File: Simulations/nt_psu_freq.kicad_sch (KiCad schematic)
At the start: 14 parts, among them Q1 DMP2008UFG

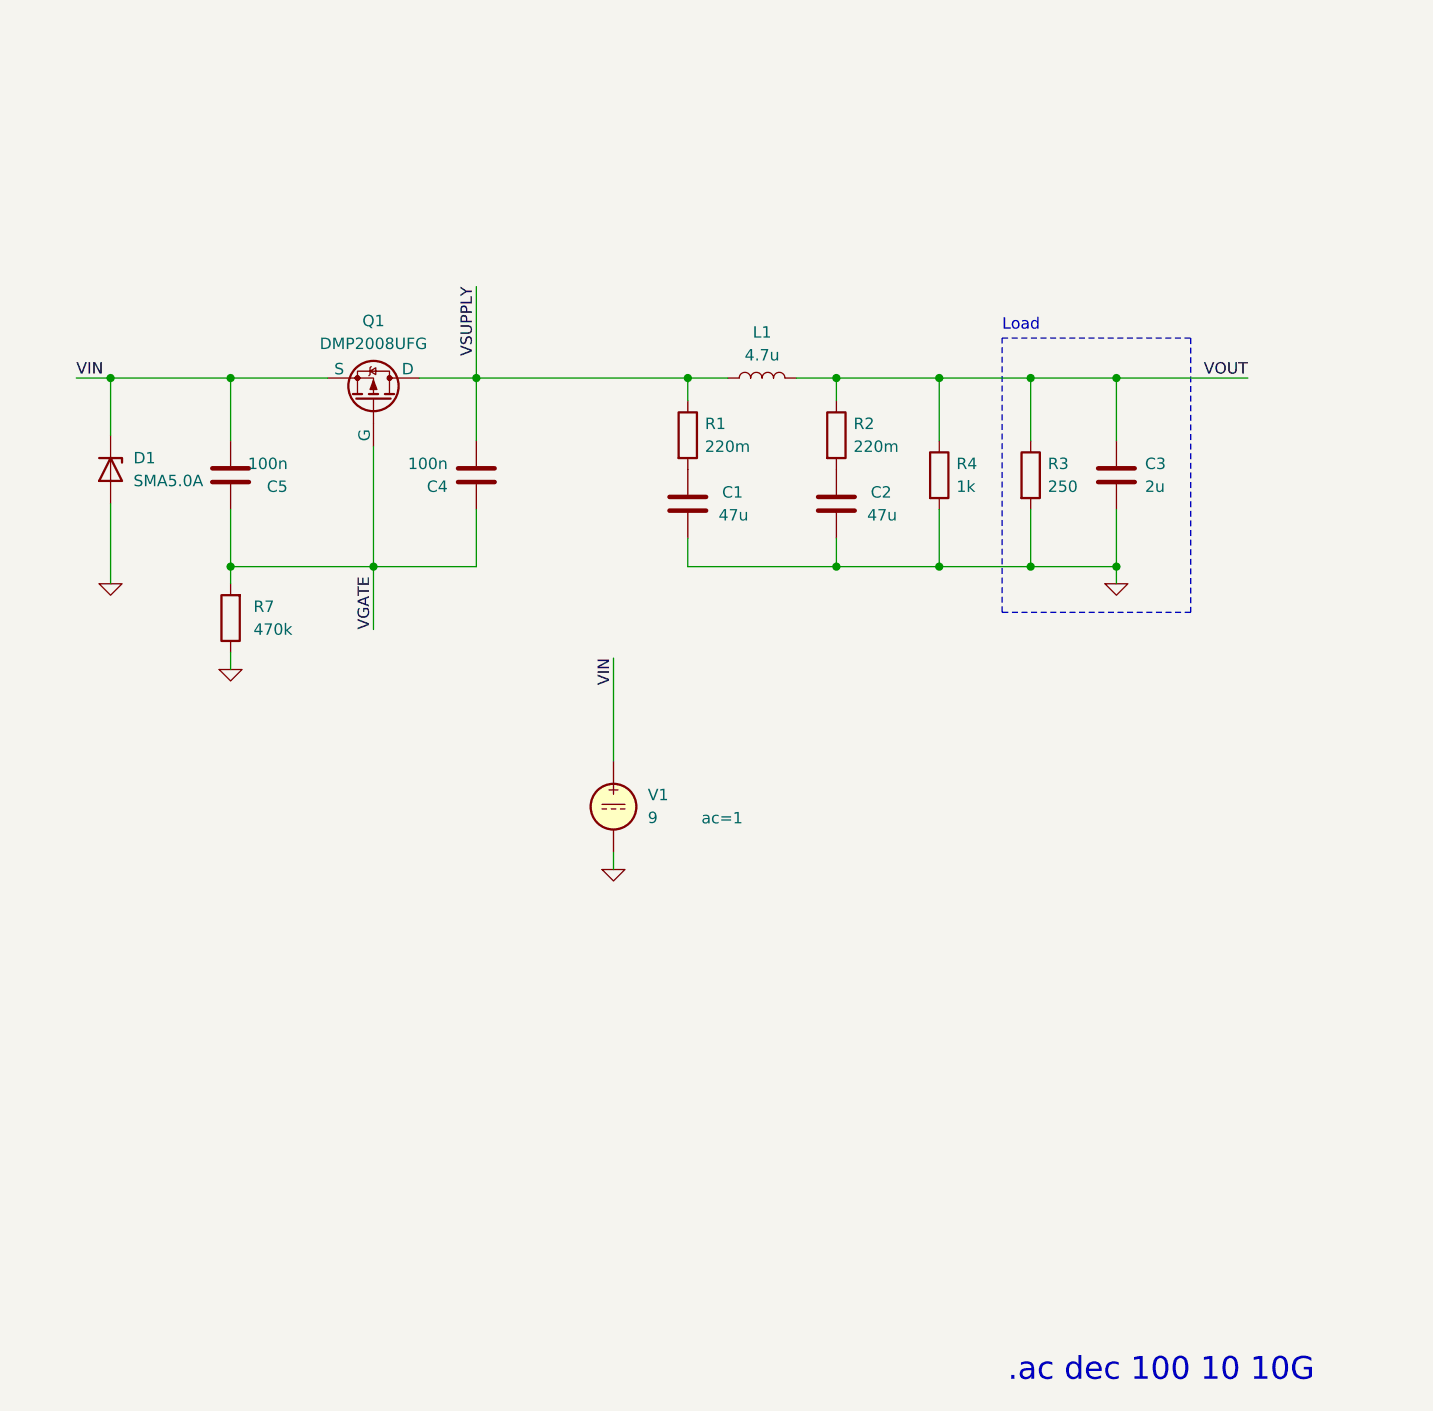
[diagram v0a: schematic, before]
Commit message: fine tuning before layout
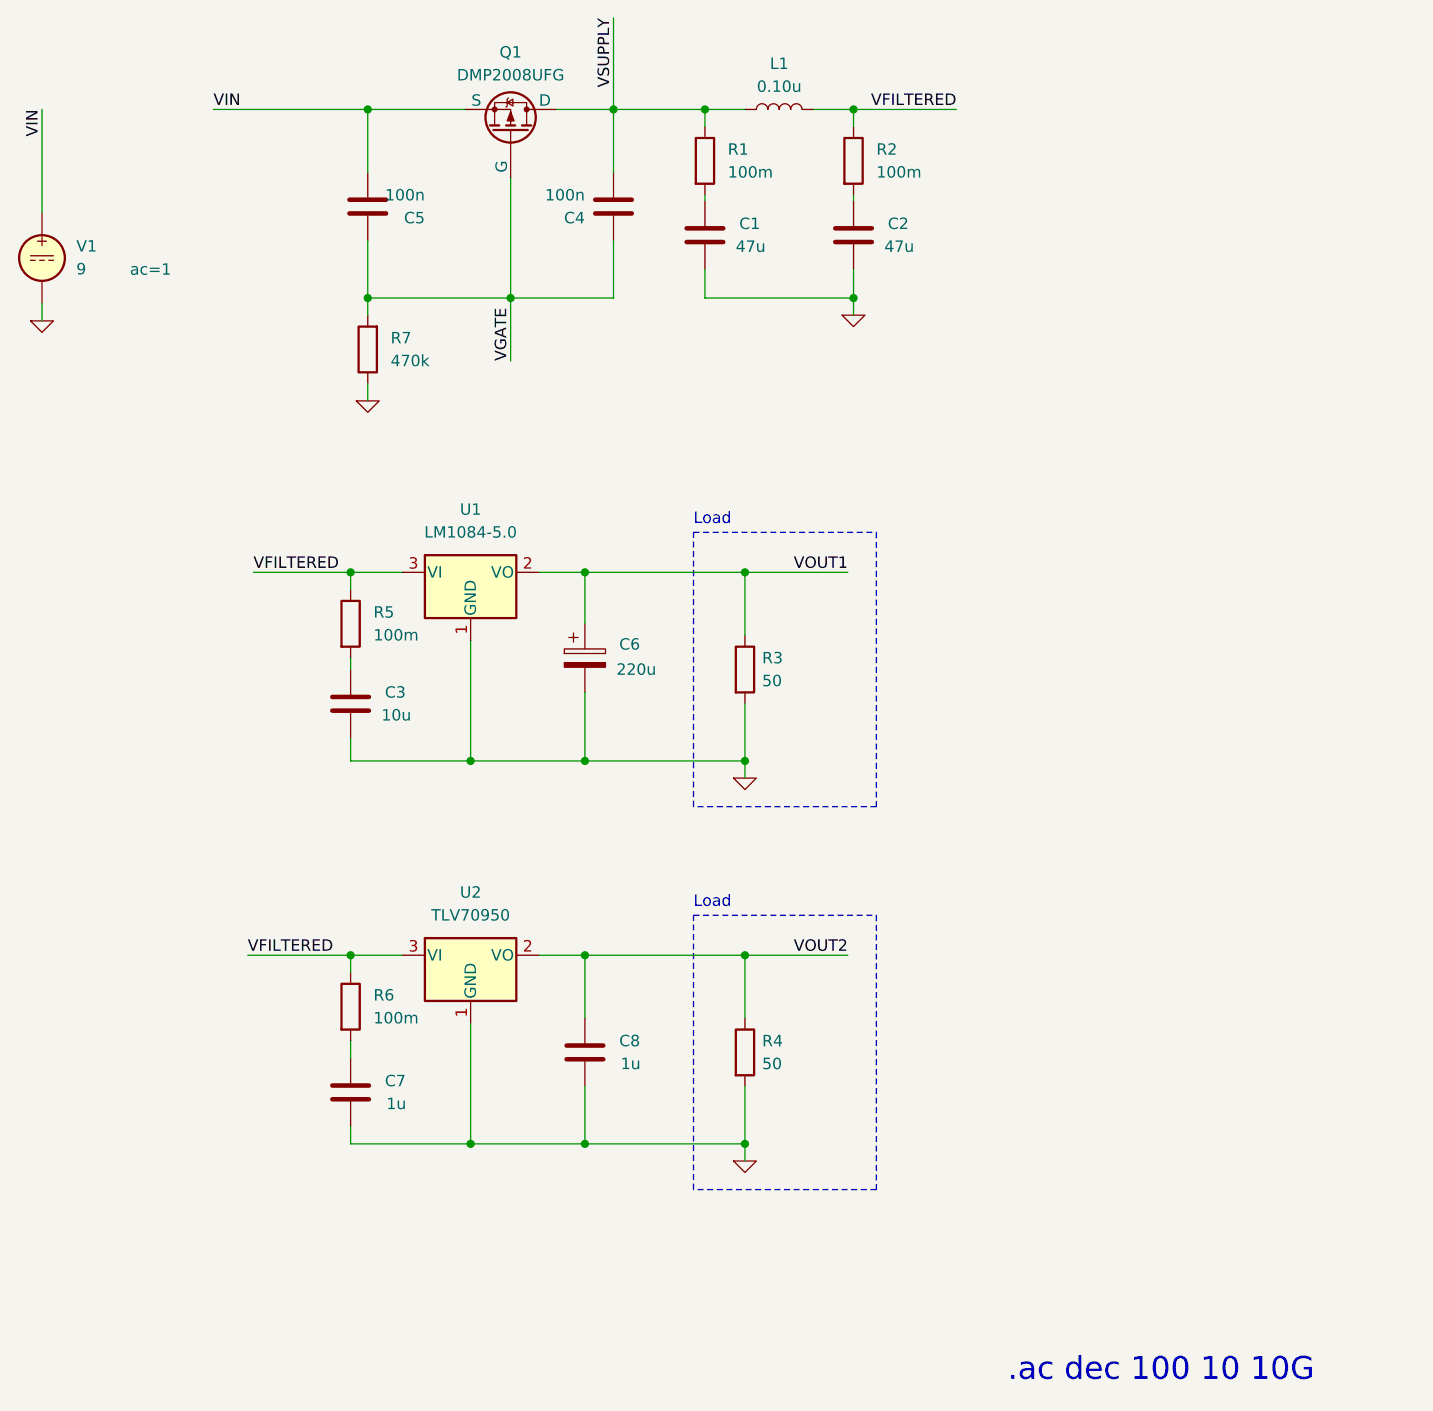
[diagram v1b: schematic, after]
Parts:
- removed D1: SMA5.0A, symbol Device:D_Zener
- added C6: ${SIM.PARAMS}, symbol Device:C_Polarized
- added C7, C8: ${SIM.PARAMS}, symbol Device:C
- added R5, R6: 100m, symbol Device:R
- added U1: LM1084-5.0, symbol Regulator_Linear:LM1084-5.0
- added U2: TLV70950, symbol Regulator_Linear:LM1084-5.0
- C3: value 2u -> ${SIM.PARAMS}
- R1, R2: value 220m -> 100m
- R3: value 250 -> 50
- R4: value 1k -> 50
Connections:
- net 0: now also C6.2, C7.2, C8.2, U1.1 (GND), U2.1 (GND)
- removed net VOUT: C3.1, L1.2, R2.1, R3.1, R4.1
- new net: C7.1, R6.2
- new net: C3.1, R5.2
- new net VFILTERED: L1.2, R2.1, R5.1, R6.1, U1.3 (VI), U2.3 (VI)
- new net VOUT1: C6.1, R3.1, U1.2 (VO)
- new net VOUT2: C8.1, R4.1, U2.2 (VO)
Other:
- moved on the sheet: C1, C4, C5, L1, Q1, R3, R7, V1
